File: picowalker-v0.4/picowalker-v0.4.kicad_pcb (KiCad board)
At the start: 4 copper layers, 47.4 x 50.5 mm, 105 parts, among them J1 12402012E212A, J2 BAT, J3 SWD, J4 UART, SW1 ~{BOOT}, SW2 RUN, SW3 BUT_M, SW4 BUT_R, SW5 BUT_L, U1 RP2350A-QFN60, U2 W25Q128JVP, U3 BMA400, U4 M95512DxMC, U5 TFBS4711, U6 BQ25628ERYKR, U7 DO0180FMST0x, U8 DT1240-04LP-7, U9 RT6150B-33GQW, Y1 ABM8-272-T3, Y2 SIT1533AI-H4-DCC-32.768E

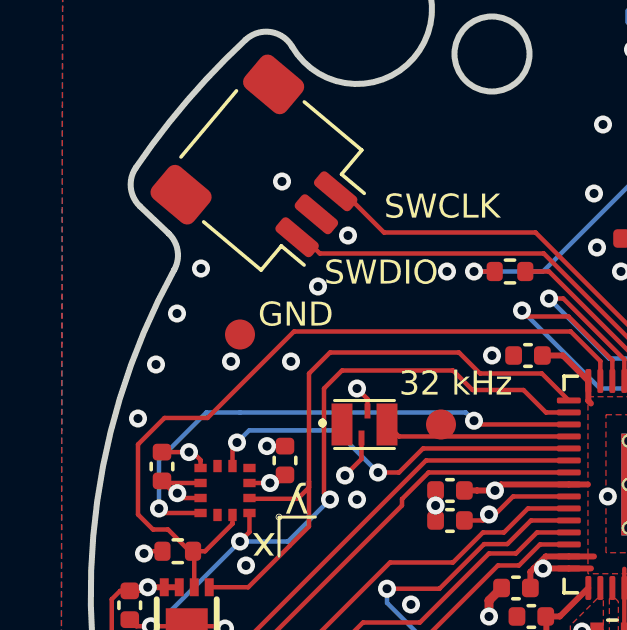
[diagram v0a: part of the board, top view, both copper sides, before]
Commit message: v0.4: send to manufacture
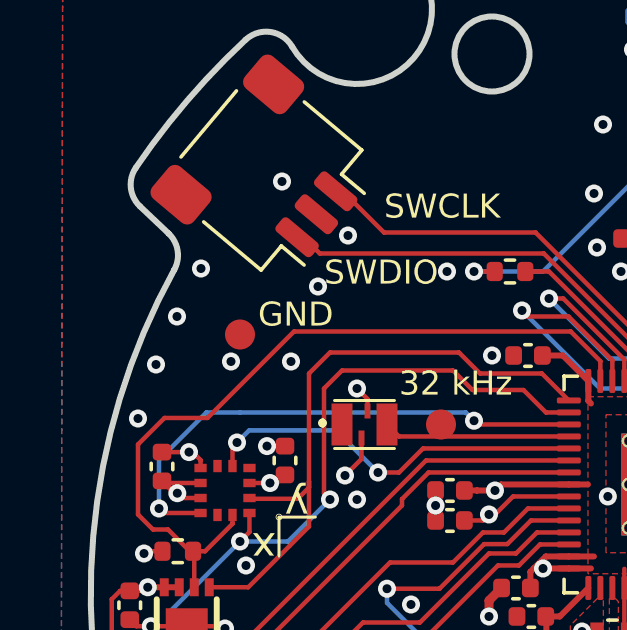
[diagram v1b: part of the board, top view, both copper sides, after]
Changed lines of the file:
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@@
 	)
 	(gr_text "Speaker"
-		(at 158.4 111.1 30)
+		(at 158.5 111.3 30)
 		(layer "B.SilkS")
 		(effects
@@
 	)
 	(via
-		(at 130.5 90.4)
-		(size 0.6)
-		(drill 0.3)
+		(at 130.5 90.5)
+		(size 0.6)
+		(drill 0.3)
